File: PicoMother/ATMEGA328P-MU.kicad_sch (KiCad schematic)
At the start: 15 parts, among them J3 M20-9980345, SW1 SW_Push, U4 ATMEGA328P-MU, Y3 Crystal_GND24

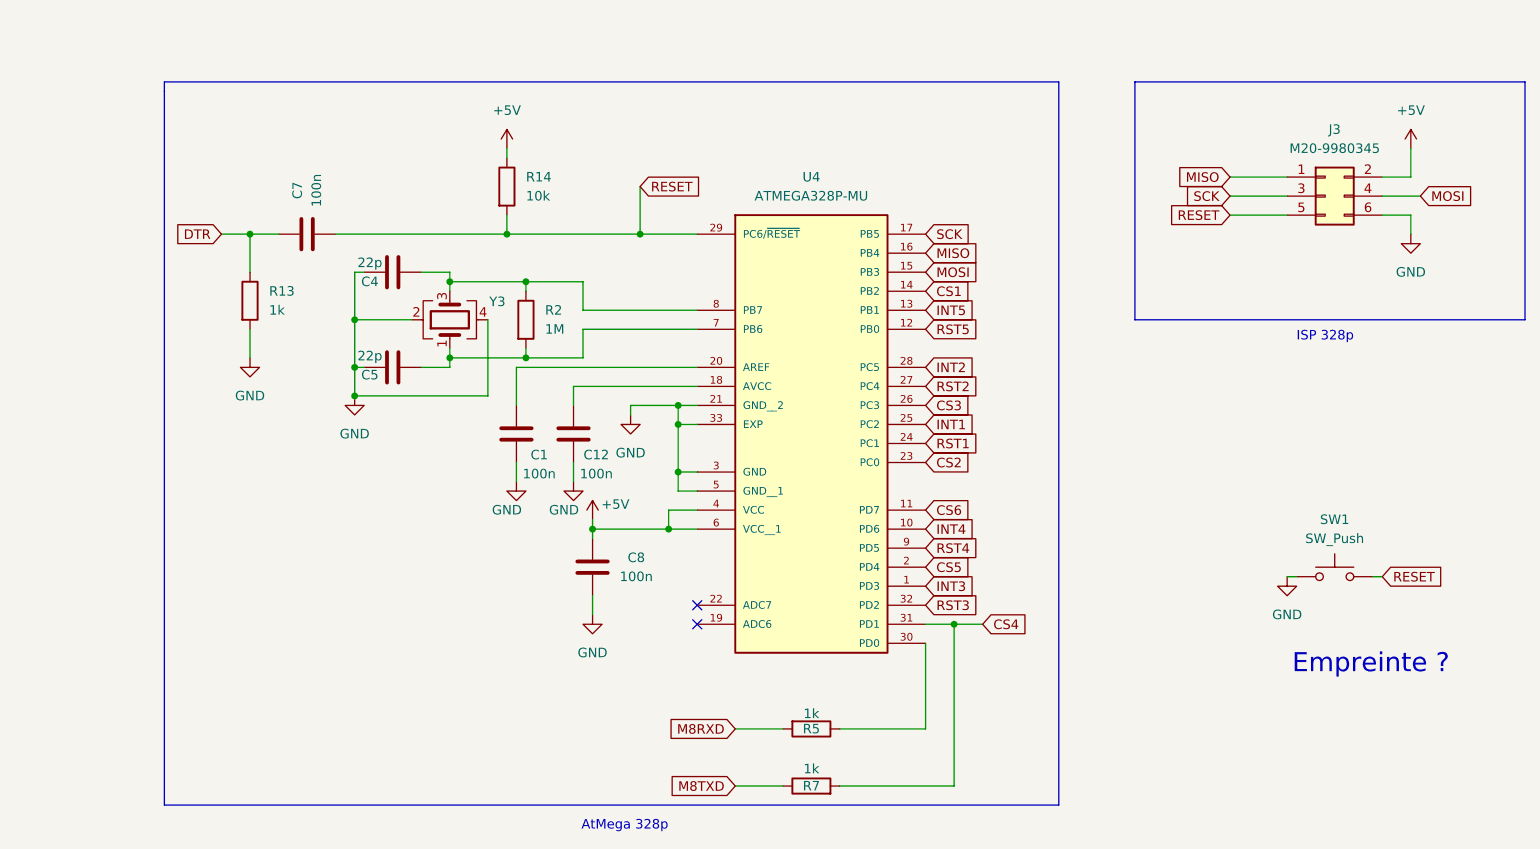
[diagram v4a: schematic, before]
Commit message: correction schematique empreintes MCU
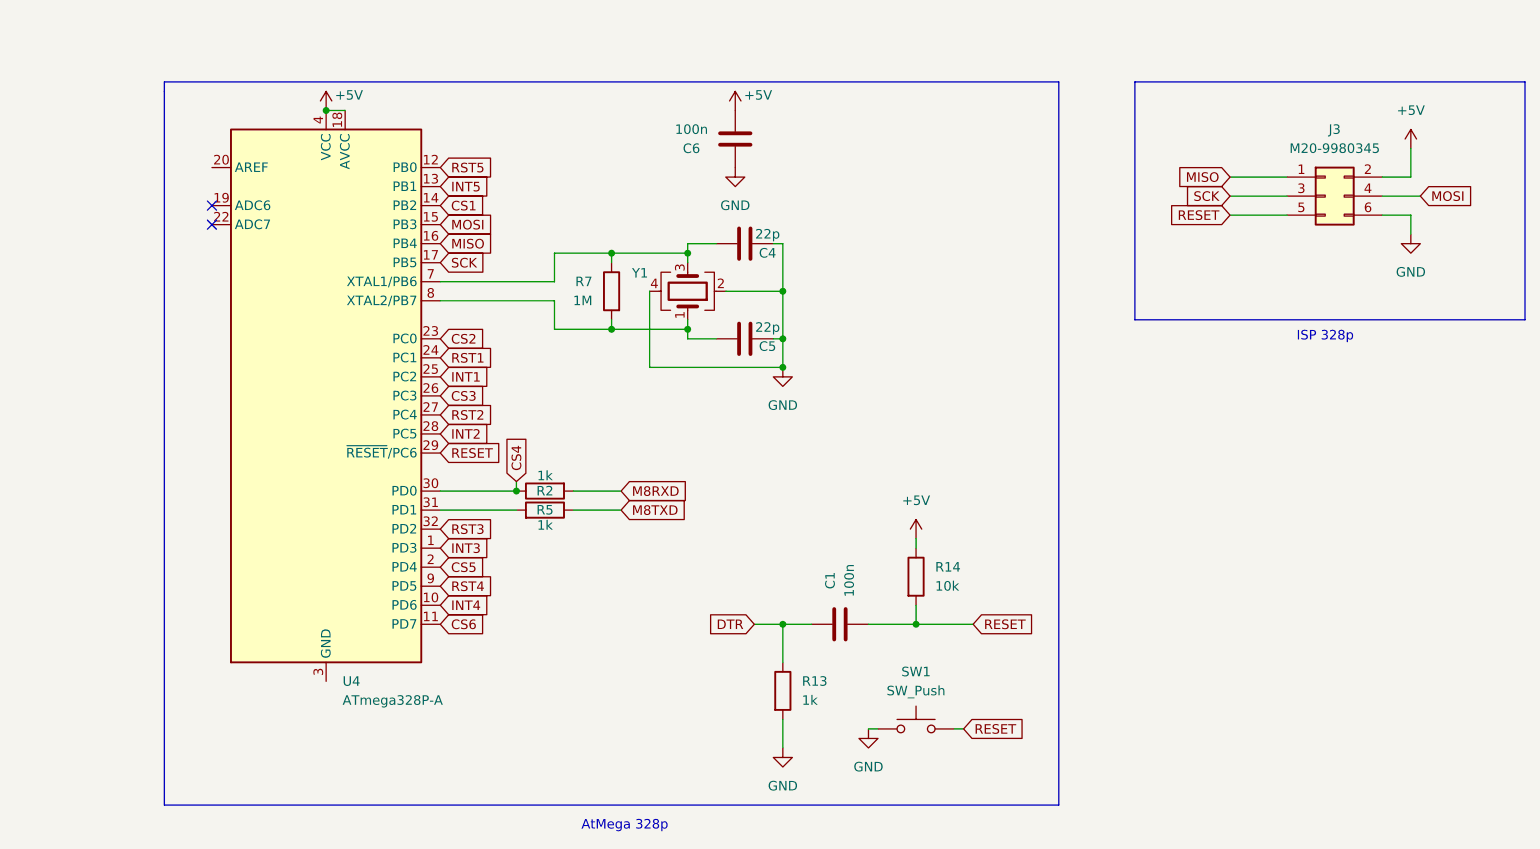
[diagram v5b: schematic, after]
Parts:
- removed C12, C7, C8: 100n, Capacitor_SMD:C_0603_1608Metric_Pad1.08x0.95mm_HandSolder, symbol Device:C
- removed U4: ATMEGA328P-MU, Package_QFP:TQFP-32_7x7mm_P0.8mm, symbol Arduino Uno SMD:ATMEGA328P-MU
- removed Y3: Crystal_GND24, Crystal:Crystal_SMD_SeikoEpson_FA238-4Pin_3.2x2.5mm_HandSoldering, symbol Device:Crystal_GND24
- added C6: 100n, Capacitor_SMD:C_0603_1608Metric_Pad1.08x0.95mm_HandSolder, symbol Device:C
- added U4: ATmega328P-A, Package_QFP:TQFP-32_7x7mm_P0.8mm, symbol MCU_Microchip_ATmega:ATmega328P-A
- added Y1: Crystal_GND24, Crystal:Crystal_SMD_SeikoEpson_FA238-4Pin_3.2x2.5mm_HandSoldering, symbol Device:Crystal_GND24
- R2: value 1M -> 1k
- R7: value 1k -> 1M
- SW1: footprint Button_Switch_THT:SW_DIP_SPSTx01_Piano_10.8x4.1mm_W7.62mm_P2.54mm -> Button_Switch_SMD:SW_Push_1P1T_NO_CK_KSC7xxJ
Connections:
- net +5V: now also C6.2, U4.18 (AVCC), U4.4 (VCC), U4.6 (VCC)
- net CS1: now also U4.14 (PB2)
- net CS2: now also U4.23 (PC0)
- net CS3: now also U4.26 (PC3)
- net CS4: now also R2.1, U4.30 (PD0); no longer R7.2
- net CS5: now also U4.2 (PD4)
- net CS6: now also U4.11 (PD7)
- net DTR: now also C1.1
- net GND: now also C6.1, Y1.2, Y1.4; no longer C1.2
- net INT1: now also U4.25 (PC2)
- net INT2: now also U4.28 (PC5)
- net INT3: now also U4.1 (PD3)
- net INT4: now also U4.10 (PD6)
- net INT5: now also U4.13 (PB1)
- net M8RXD: now also R2.2; no longer R5.2
- net M8TXD: now also R5.1; no longer R7.1
- net MISO: now also U4.16 (PB4)
- net MOSI: now also U4.15 (PB3)
- net RESET: now also C1.2, U4.29 (~{RESET}/PC6)
- net RST1: now also U4.24 (PC1)
- net RST2: now also U4.27 (PC4)
- net RST3: now also U4.32 (PD2)
- net RST4: now also U4.9 (PD5)
- net RST5: now also U4.12 (PB0)
- net SCK: now also U4.17 (PB5)
- net at C4.1: now also R7.1, U4.7 (XTAL1/PB6), Y1.3; no longer R2.1
- net at C5.1: now also R7.2, U4.8 (XTAL2/PB7), Y1.1; no longer R2.2
- new net: U4.21 (GND), U4.3 (GND), U4.5 (GND)
- new net: R5.2, U4.31 (PD1)
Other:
- note removed: "Empreinte ?"

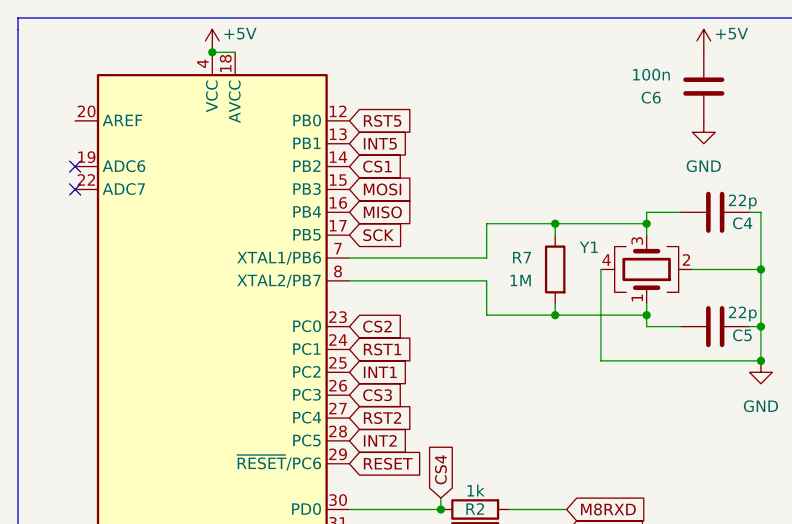
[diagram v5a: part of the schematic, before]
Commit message: début de routage, premiers changement d'E/S sur le 328 pour faciliter le routage
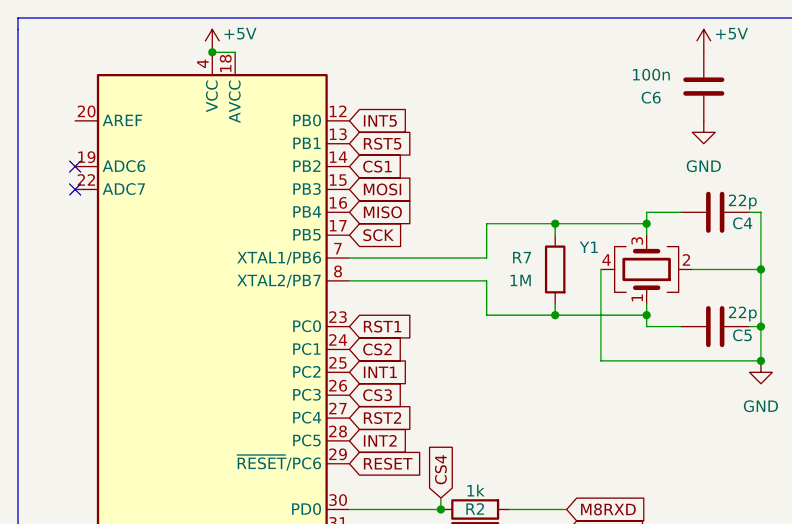
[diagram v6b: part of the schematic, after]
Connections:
- net CS2: now also U4.24 (PC1); no longer U4.23 (PC0)
- net INT5: now also U4.12 (PB0); no longer U4.13 (PB1)
- net RST1: now also U4.23 (PC0); no longer U4.24 (PC1)
- net RST5: now also U4.13 (PB1); no longer U4.12 (PB0)

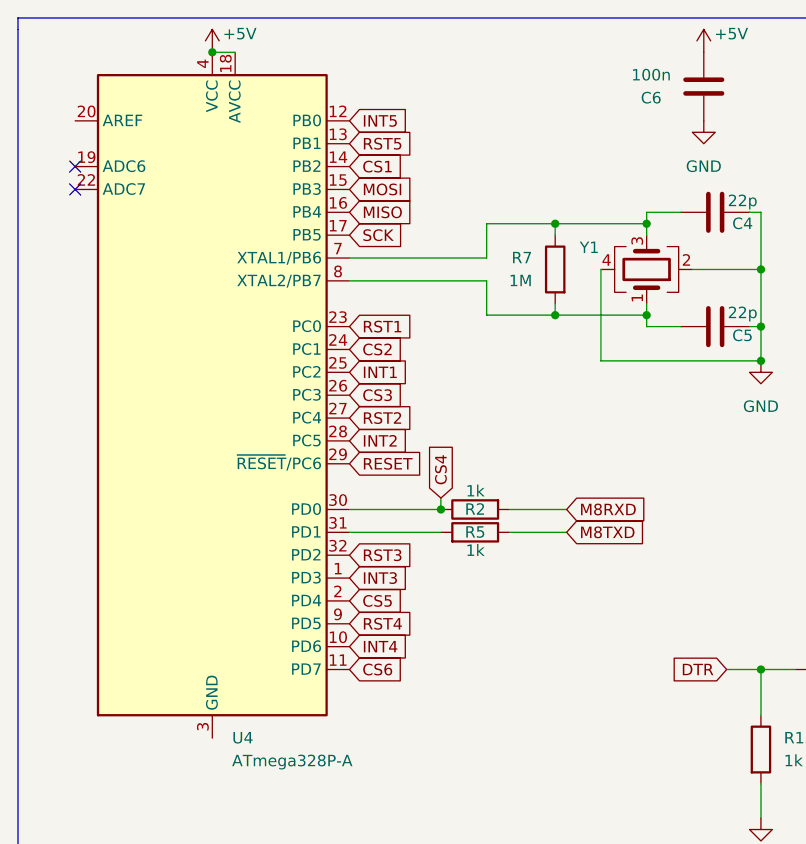
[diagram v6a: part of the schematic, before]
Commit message: routage bien avancé, derniers changement d'E/S sur le 328 pour faciliter le routage
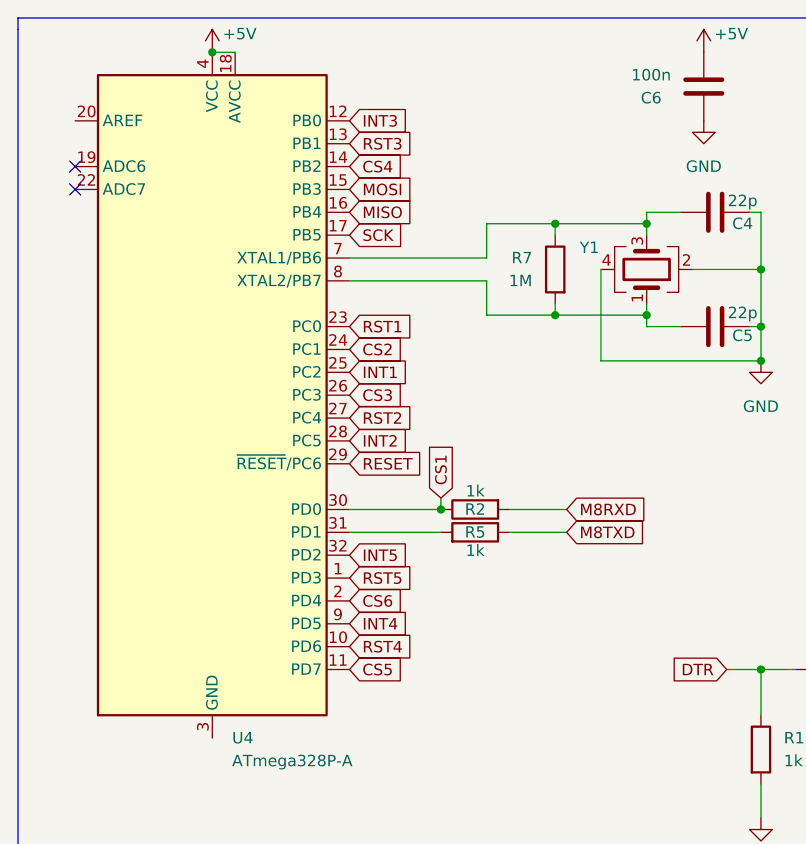
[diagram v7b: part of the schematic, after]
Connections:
- net CS1: now also R2.1, U4.30 (PD0); no longer U4.14 (PB2)
- net CS4: now also U4.14 (PB2); no longer R2.1, U4.30 (PD0)
- net CS5: now also U4.11 (PD7); no longer U4.2 (PD4)
- net CS6: now also U4.2 (PD4); no longer U4.11 (PD7)
- net INT3: now also U4.12 (PB0); no longer U4.1 (PD3)
- net INT4: now also U4.9 (PD5); no longer U4.10 (PD6)
- net INT5: now also U4.32 (PD2); no longer U4.12 (PB0)
- net RST3: now also U4.13 (PB1); no longer U4.32 (PD2)
- net RST4: now also U4.10 (PD6); no longer U4.9 (PD5)
- net RST5: now also U4.1 (PD3); no longer U4.13 (PB1)
